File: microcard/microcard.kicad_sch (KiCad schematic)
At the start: 32 parts, among them CN1 HC-1.2-4PWT, J1 Conn_01x08, J2 CHG, Q1 2N7002, SW1 BOOT, SW2 SEL, SW3 ESC, SW4 UP, SW5 DWN, SW6 TRG, SW7 DIM, SW8 RST, U1 ESP32-WROOM-32UE

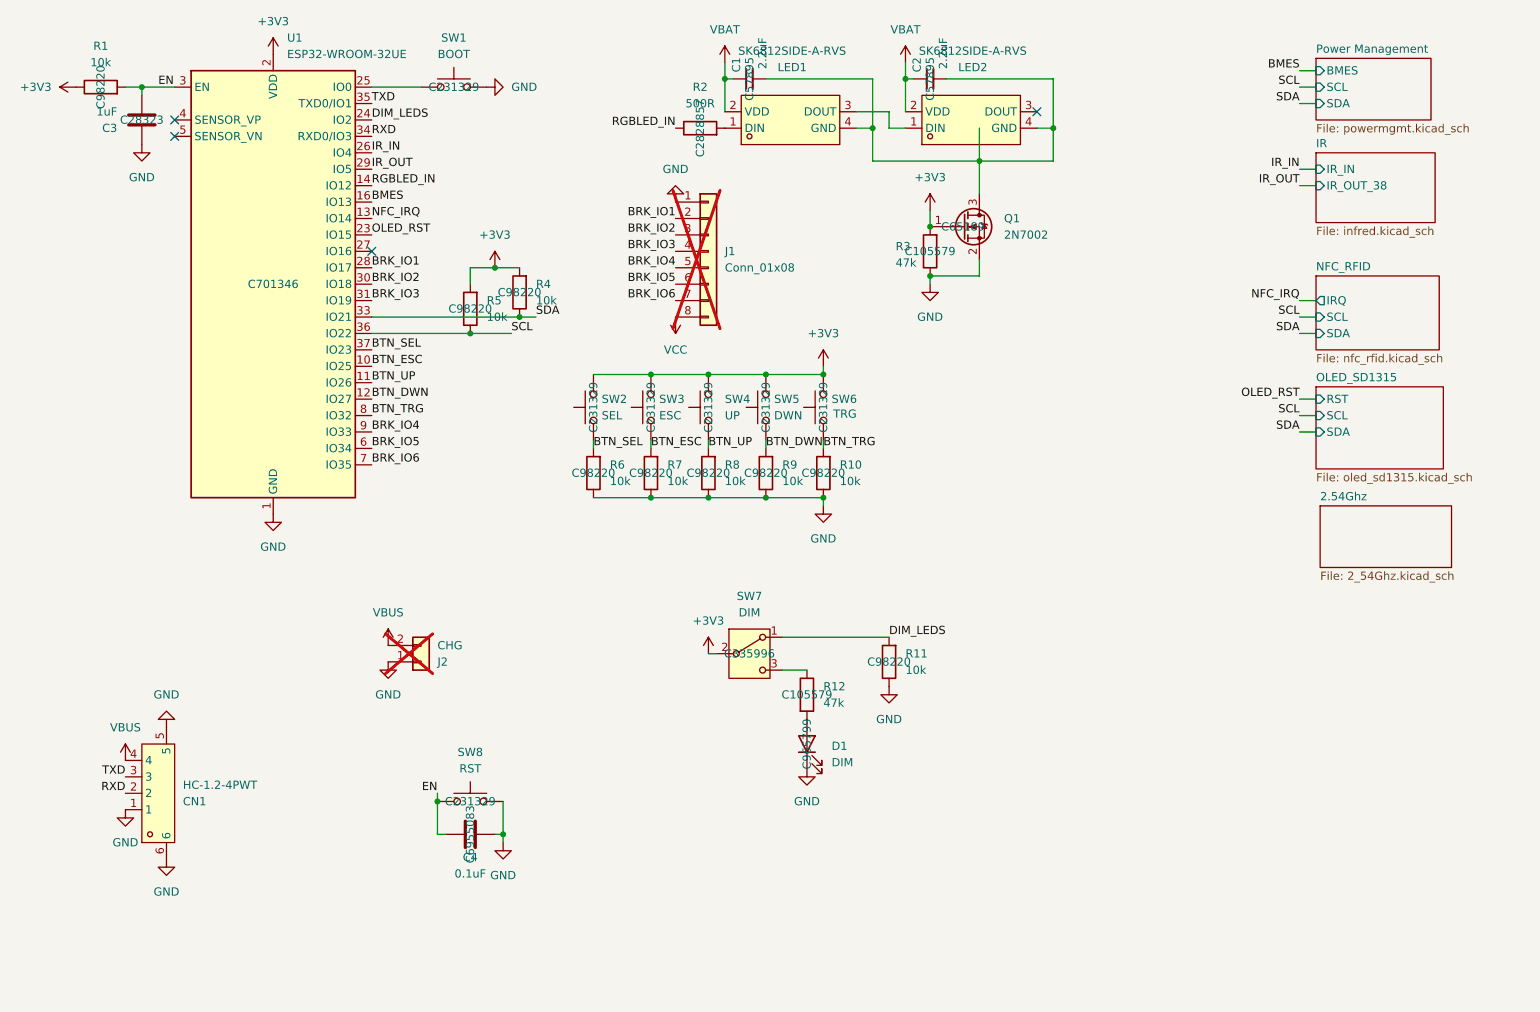
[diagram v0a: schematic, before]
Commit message: wide render
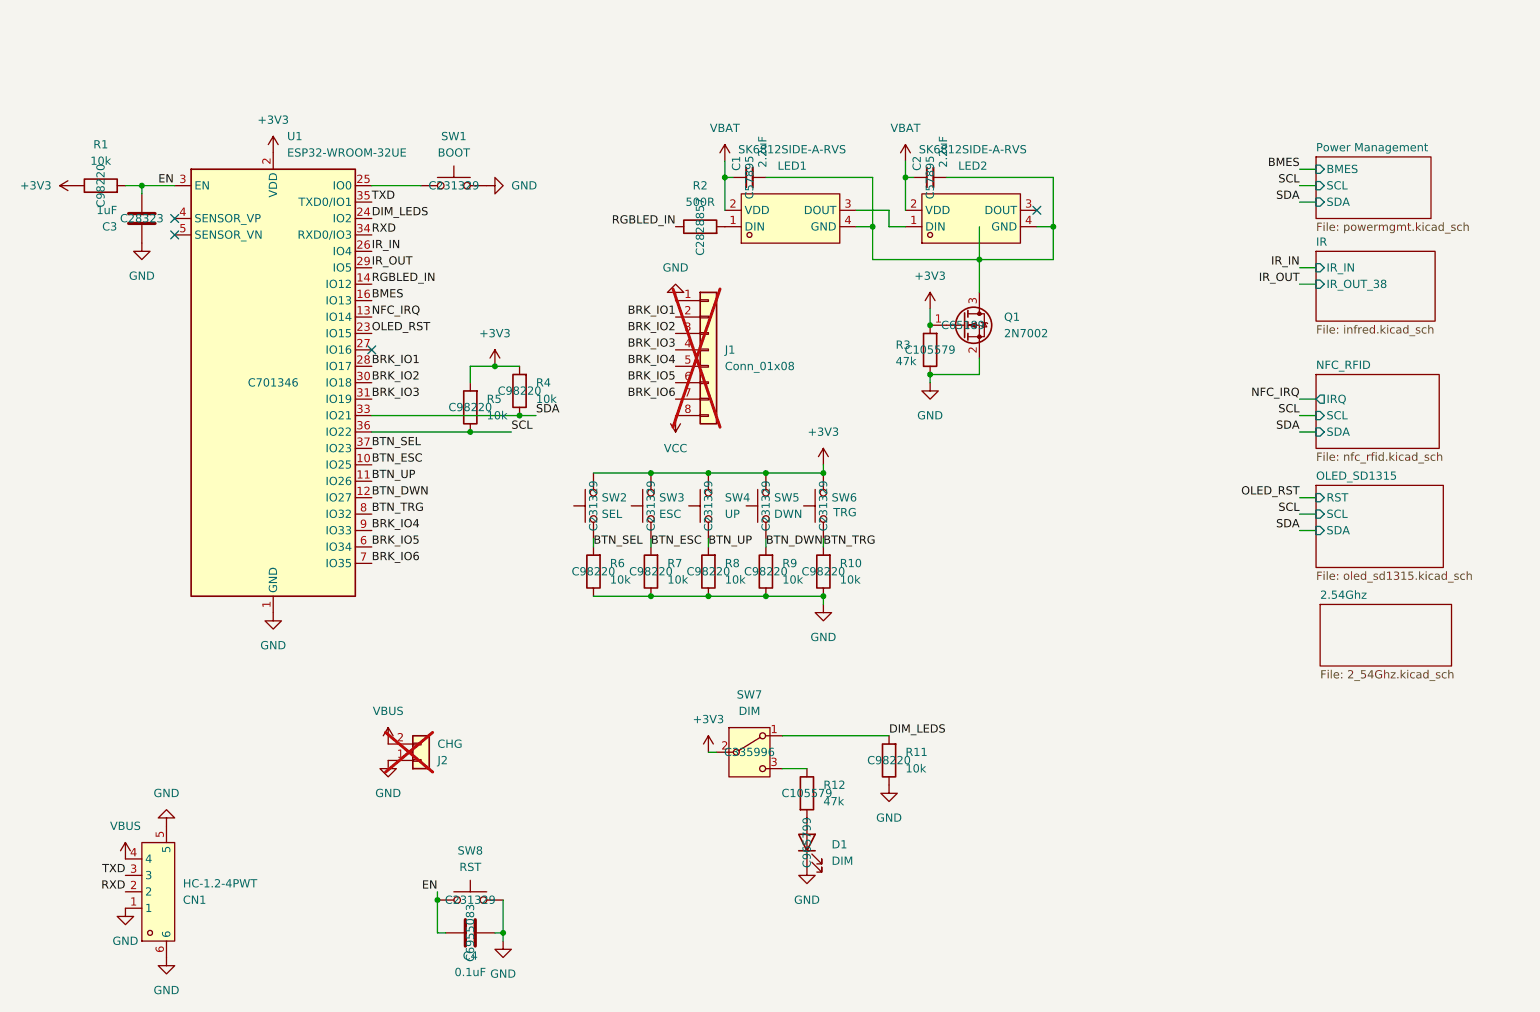
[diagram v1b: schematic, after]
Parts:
- C1, C2, C4: footprint Capacitor_SMD:C_0603_1608Metric_Pad1.08x0.95mm_HandSolder -> Capacitor_SMD:C_0603_1608Metric
- C3: footprint Capacitor_SMD:C_0805_2012Metric_Pad1.18x1.45mm_HandSolder -> Capacitor_SMD:C_0805_2012Metric
- D1: footprint Diode_SMD:D_0603_1608Metric_Pad1.05x0.95mm_HandSolder -> Diode_SMD:D_0603Metric
- R1, R10, R11, R12, R3, R4, R5, R6, R7, R8, R9: footprint Resistor_SMD:R_0603_1608Metric_Pad0.98x0.95mm_HandSolder -> Resistor_SMD:R_0603_1608Metric
- R2: footprint Resistor_SMD:R_0805_2012Metric_Pad1.20x1.40mm_HandSolder -> Resistor_SMD:R_0805_2012Metric
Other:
- moved on the sheet: C1, C2, C3, C4, CN1, D1, J1, J2, LED1, LED2, Q1, R1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
